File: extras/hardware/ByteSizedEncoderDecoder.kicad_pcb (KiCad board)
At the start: 2 copper layers, 21.6 x 25.4 mm, 17 parts, among them J1 SM04B-SRSS-TB, J10 1x4 female header pins 0.1", J11 ICSP pads (for interfacing wi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, J2 SM04B-SRSS-TB, J3 1x4 female header pins 0.1", J4 1x4 female header pins 0.1", J5 1x4 female header pins 0.1", J6 1x4 female header pins 0.1", J7 1x4 female header pins 0.1", J8 1x4 female header pins 0.1", J9 1x4 female header pins 0.1", U1 ATMEGA328PB, 32-TQFP

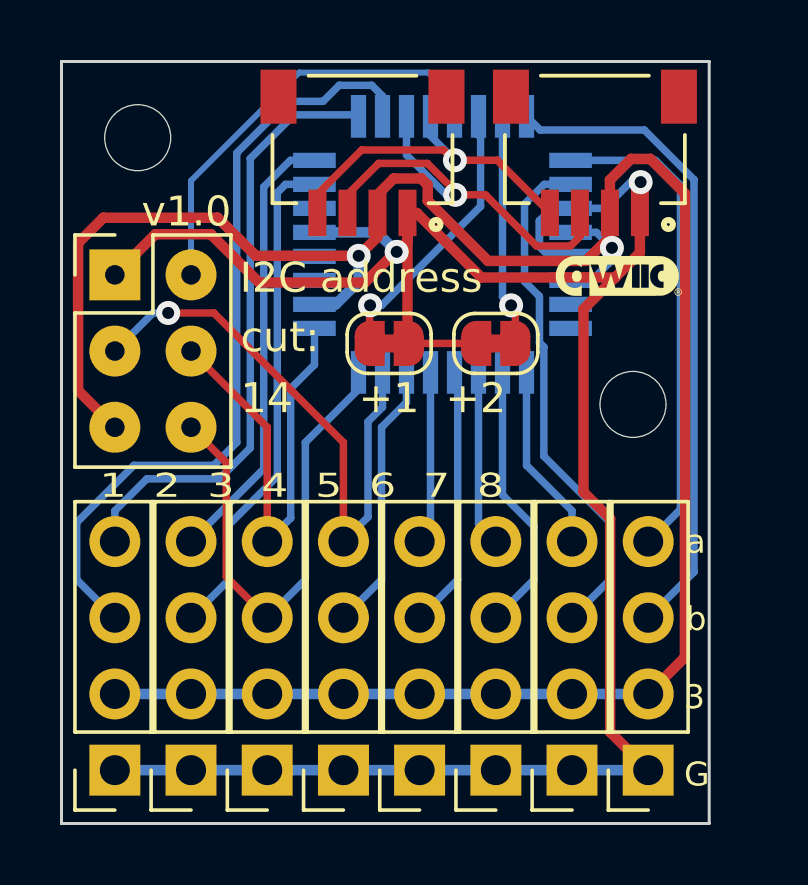
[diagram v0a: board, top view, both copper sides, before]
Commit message: v1.1.0
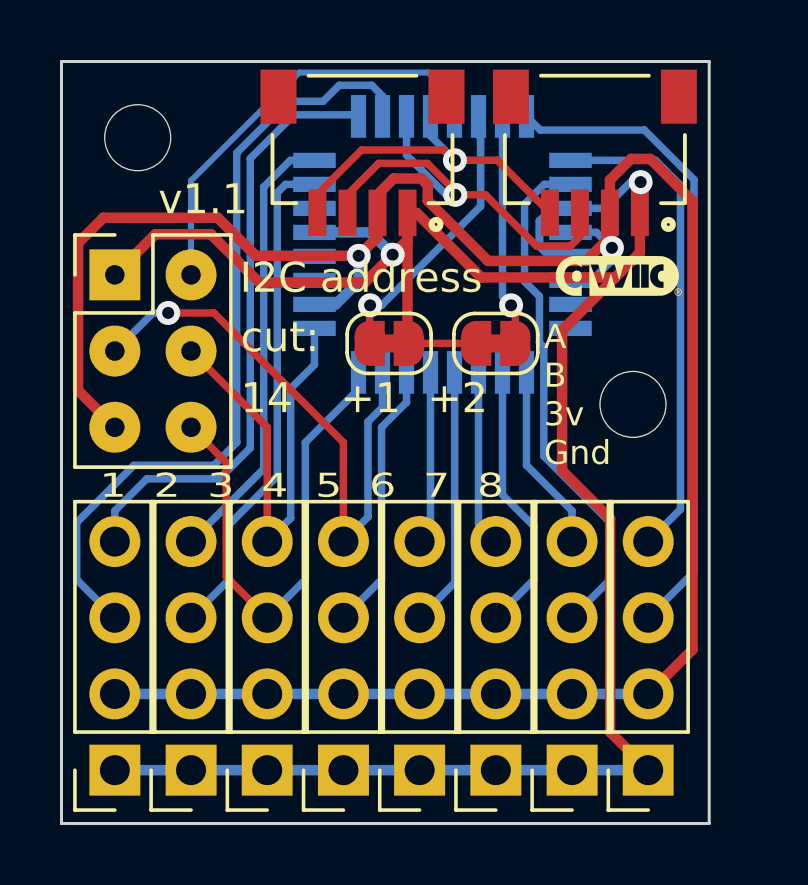
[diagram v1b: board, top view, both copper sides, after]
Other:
- board text added: "A B 3v Gnd"
- board text added: "v1.1"
- board text removed: "3 G"
- board text removed: "a b"
- board text removed: "v1.0"
